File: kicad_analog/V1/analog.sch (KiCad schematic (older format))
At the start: 29 parts, among them P1 Conn_02x05_Odd_Even, P2 Conn_01x04, P3 Conn_01x05, P4 Conn_01x02, P6 Conn_01x01, P7 Conn_01x01, U1 MAX9144, U2 MAX9144, U4 MCP1754S-3302xCB, U5 TS5A3166DBVR

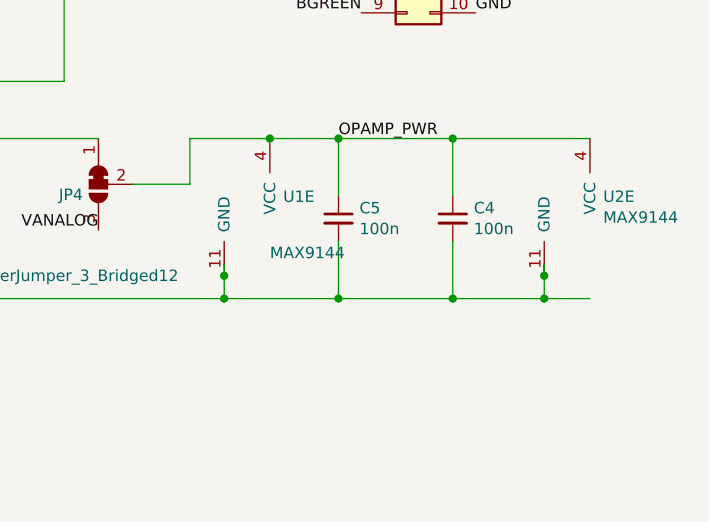
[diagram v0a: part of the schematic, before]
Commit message: Issue 2 analog board part2
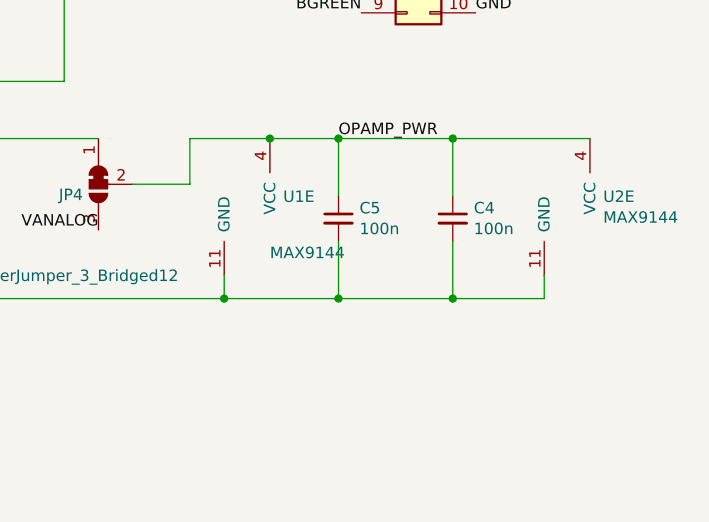
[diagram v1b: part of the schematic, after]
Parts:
- UB1: footprint (none) -> Package_SO:VSSOP-10_3x3mm_P0.5mm
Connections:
- wire segments 175 -> 172
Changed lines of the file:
@@
 Wire Wire Line
 	4850 6700 4950 6700
-Connection ~ 10150 6450
 Connection ~ 7400 6450
 Wire Wire Line
@@
 Wire Wire Line
 	9350 5750 9650 5750
-Wire Wire Line
-	9150 6300 9150 6350
 Connection ~ 9150 6450
 Wire Wire Line
 	9150 6450 9650 6450
-Connection ~ 9150 6350
 Wire Wire Line
 	9150 6350 9150 6450
@@
 	1    0    0    -1
 $EndComp
-Wire Wire Line
-	10550 6300 10550 6350
-Wire Wire Line
-	10150 6450 10550 6450
-Wire Wire Line
-	10550 6350 10550 6450
-Connection ~ 10550 6350
-Connection ~ 10550 6450
-Wire Wire Line
-	10550 6450 10750 6450
 $Comp
 L Device:C_Small C6
@@
 F 0 "UB1" H 2900 7515 50  0000 C CNN
 F 1 "DAC084S085" H 2900 7424 50  0000 C CNN
-F 2 "" H 2900 6950 50  0001 C CNN
+F 2 "Package_SO:VSSOP-10_3x3mm_P0.5mm" H 2900 6950 50  0001 C CNN
 F 3 "" H 2900 6950 50  0001 C CNN
 	1    2900 6950
@@
 Wire Wire Line
 	2400 6200 3400 6200
+Connection ~ 10150 6450
+Wire Wire Line
+	10550 6350 10550 6450
+Wire Wire Line
+	10150 6450 10550 6450
 $EndSCHEMATC
